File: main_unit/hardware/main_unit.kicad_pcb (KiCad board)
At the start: 4 copper layers, 75 x 65 mm, 82 parts, among them J1 62684-402100ALF, J2 Conn_02x07_Odd_Even, J3 691137710002, J4 691137710002, Q1 2N7002BK,215, SW1 PTS636SM43SMTR LFS, U1 STM32H753ZIT6, U2 LD39200PU33R, U3 W9864G6KH-6, U4 MAX25512ATG/V+T, U5 ATA6561-GAQW-N, Y1 ABM8G-25.000MHZ-18-D2Y-T, Y2 SC32S-7PF20PPM

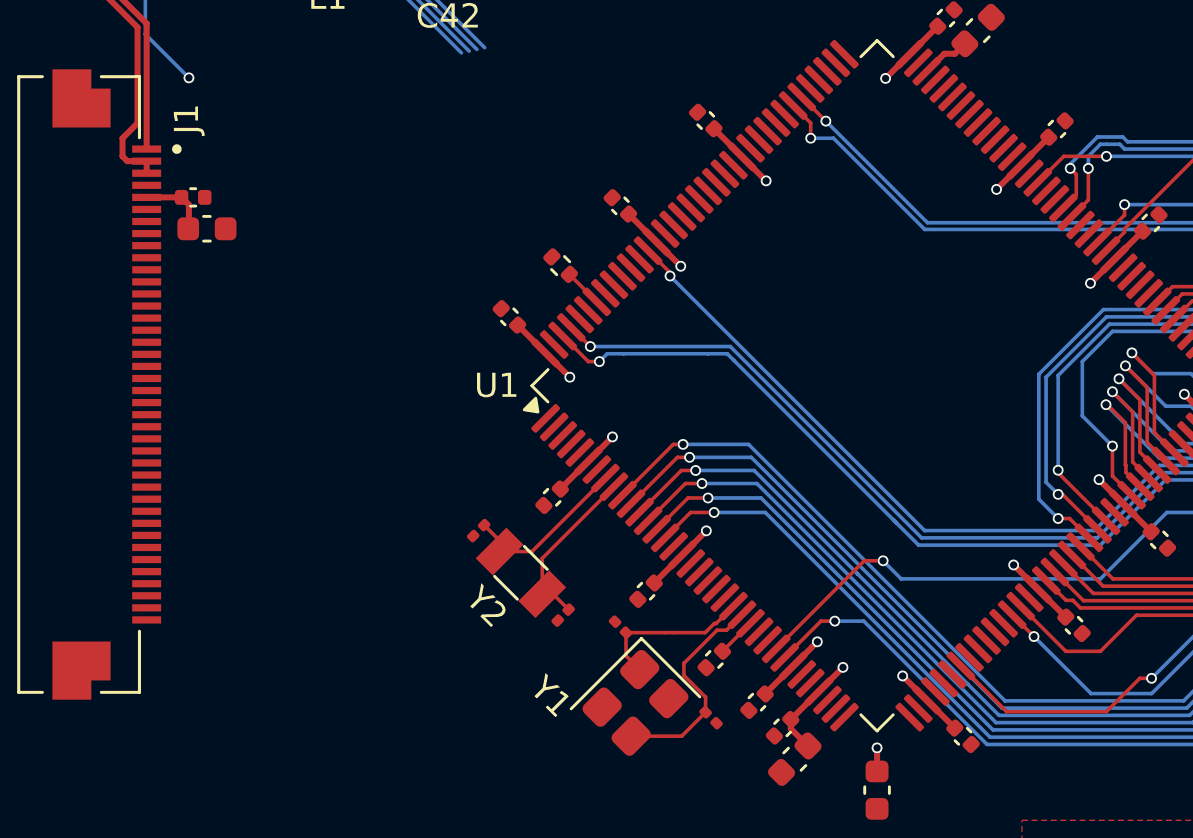
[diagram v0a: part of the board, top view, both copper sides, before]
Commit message: main_unit/hardware: Route out control signals for LCD
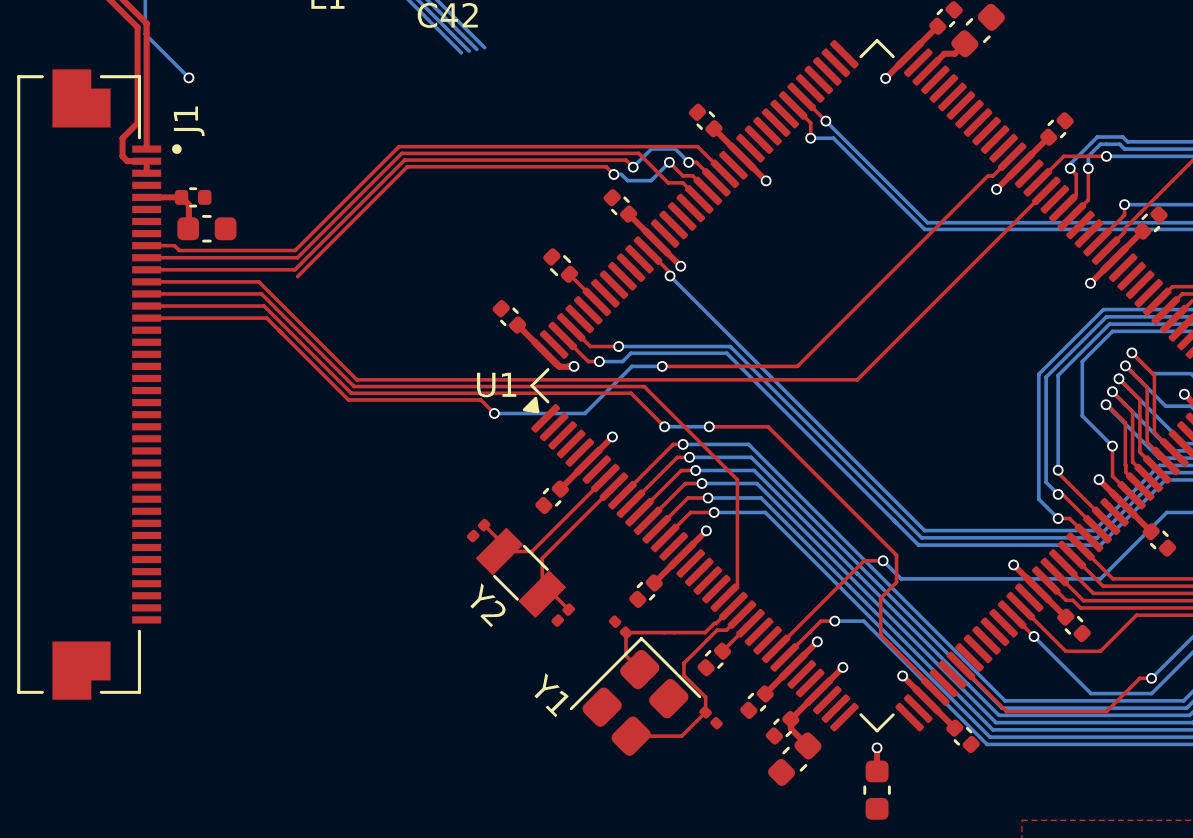
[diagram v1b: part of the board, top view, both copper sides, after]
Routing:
- net LCD_VSYNC: track 0.00 -> 42.2 mm, vias 0 -> 2
- net LCD_CLK: track 0.00 -> 42.2 mm
- net LCD_HSYNC: track 0.00 -> 42.1 mm, vias 0 -> 2
- net LCD_DE: track 0.00 -> 32.8 mm
- net LCD_CS: track 0.00 -> 26.5 mm, vias 0 -> 2
- net LCDSPI_SDA: track 0.00 -> 26.3 mm
- net LCDSPI_SCK: track 0.00 -> 25.5 mm
- net LCD_G3: track 0.00 -> 19.9 mm, vias 0 -> 2
